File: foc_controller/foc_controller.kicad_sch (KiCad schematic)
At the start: 46 parts, among them J1 Conn_01x02, J1-Programmer1 Conn_01x05, J2 Conn_01x04, J3 Conn_01x03, J5 USB_C_Receptacle_USB2.0_16P, J6 Conn_01x02, U1 AZ1117-3.3, U2 INA4180A2IPWR, U4 AS5048B, U5 STM32G431KBUx, Y1 16MHz

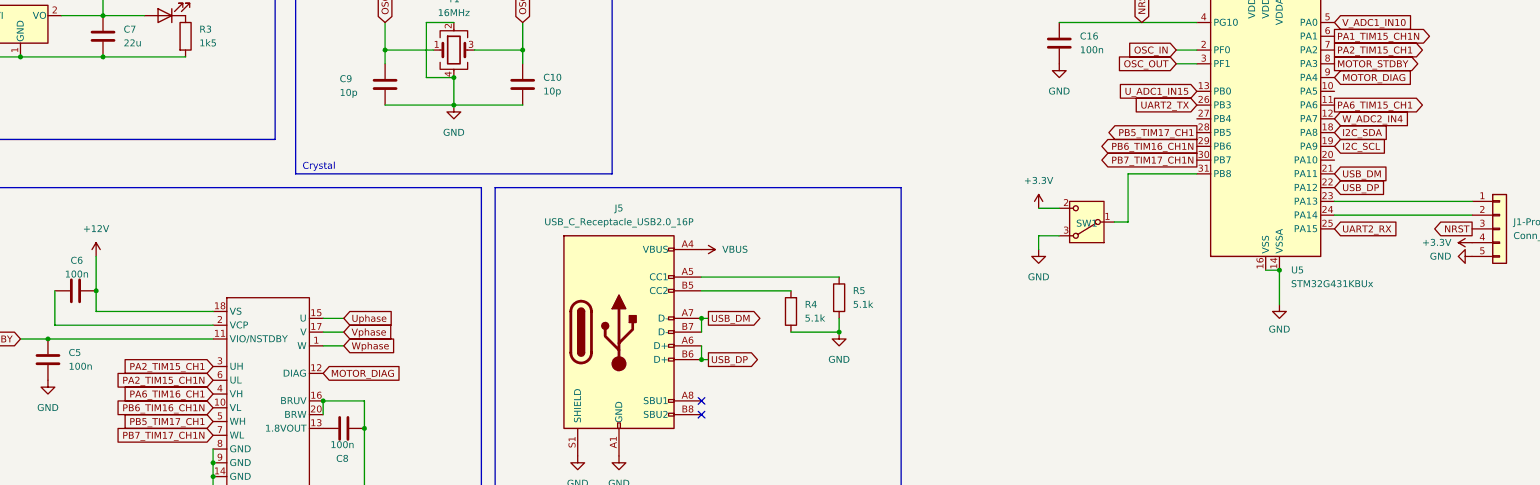
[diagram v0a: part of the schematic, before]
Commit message: Commiting again
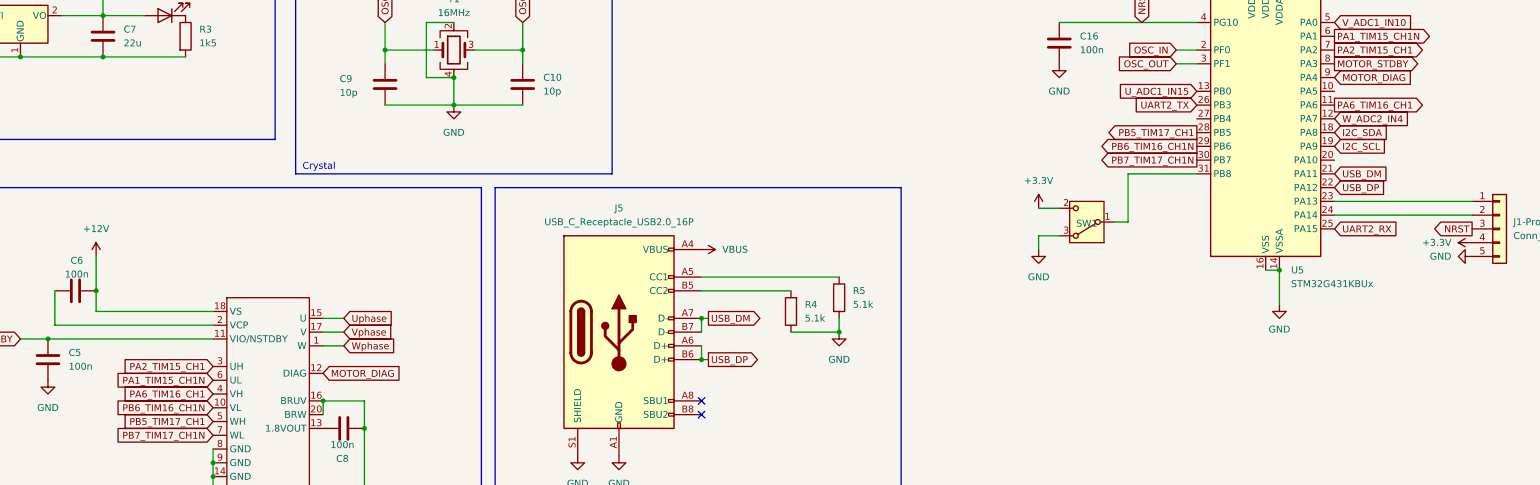
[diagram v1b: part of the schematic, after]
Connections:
- net PA2_TIM15_CH1N is gone; now on net PA1_TIM15_CH1N: U3.6 (UL)
- net PA6_TIM15_CH1 is gone; now on net PA6_TIM16_CH1: U5.11 (PA6)
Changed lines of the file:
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@@
 		)
 	)
-	(global_label "PA2_TIM15_CH1N"
+	(global_label "PA1_TIM15_CH1N"
 		(shape input)
 		(at 72.39 123.19 180)
@@
 		)
 	)
-	(global_label "PA6_TIM15_CH1"
+	(global_label "PA6_TIM16_CH1"
 		(shape output)
 		(at 279.4 72.39 0)
